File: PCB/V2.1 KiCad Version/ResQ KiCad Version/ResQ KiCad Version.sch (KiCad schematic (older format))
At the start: 7 parts, among them J1 Spare 1, J2 Spare 2, J3 OLED, J4 SD Card, J5 GPS, U1 WeMos_D1_mini

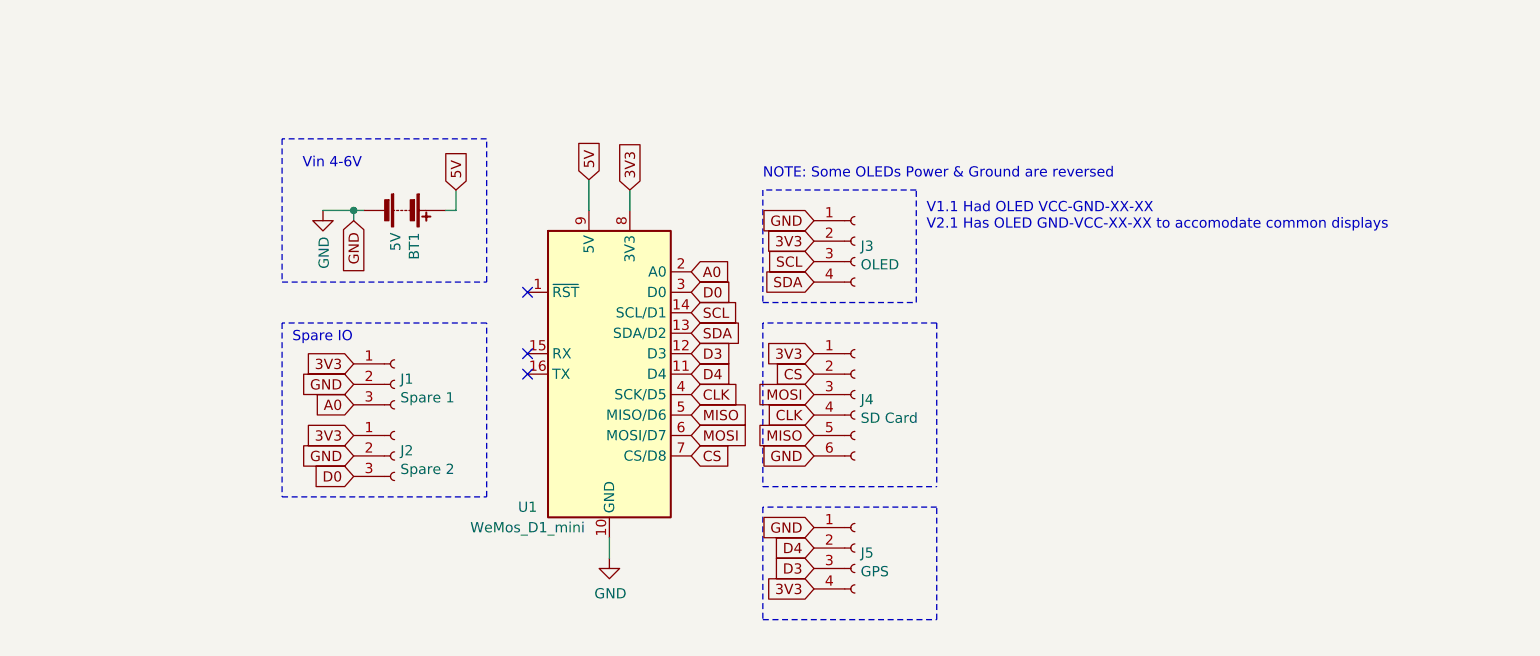
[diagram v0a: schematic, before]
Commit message: Purdier schematic
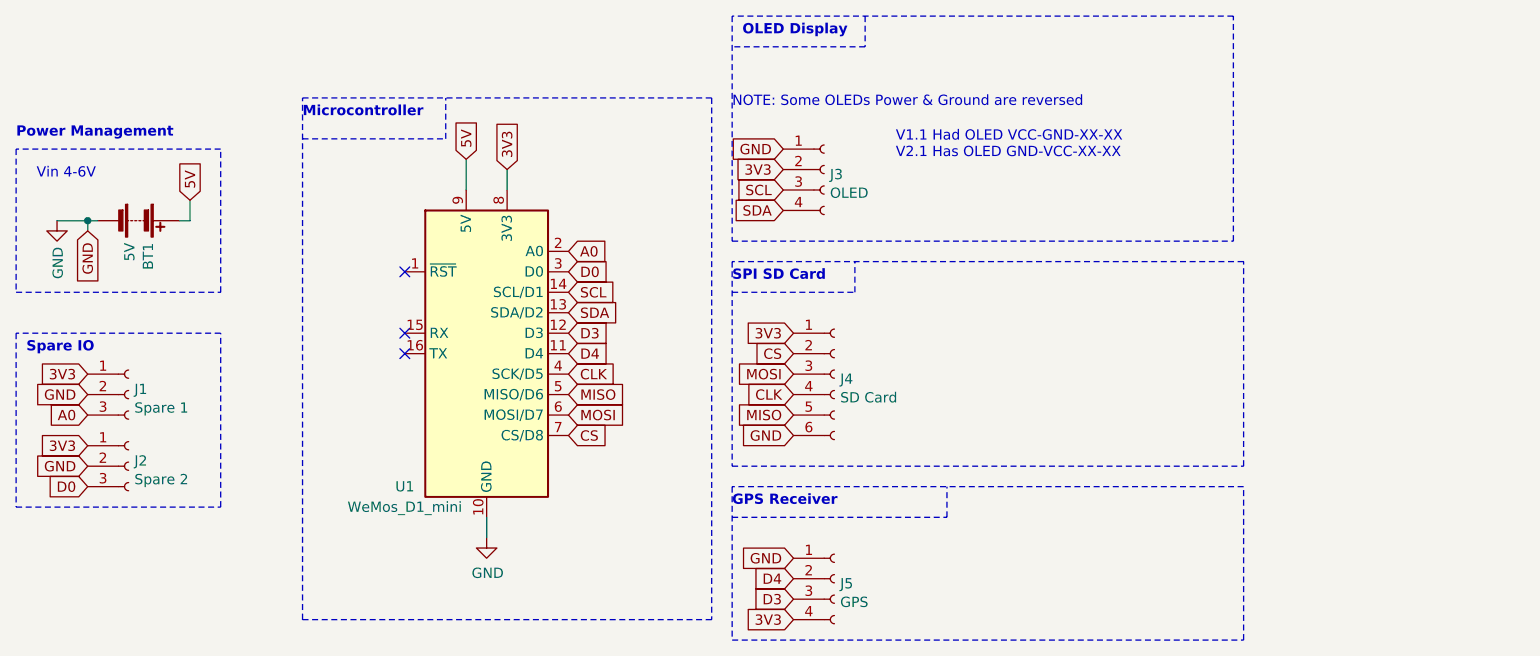
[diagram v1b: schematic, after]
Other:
- note added: "GPS Receiver"
- note added: "Microcontroller"
- note added: "OLED Display"
- note added: "Power Management"
- note added: "SPI SD Card"
- note added: "V1.1 Had OLED VCC-GND-XX-XX\nV2.1 Has OLED GND-VCC-XX-XX \n"
- note removed: "V1.1 Had OLED VCC-GND-XX-XX\nV2.1 Has OLED GND-VCC-XX-XX to accomodate common displays\n"
- moved on the sheet: BT1, J1, J2, J3, J4, J5, U1

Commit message: Purdy schematico
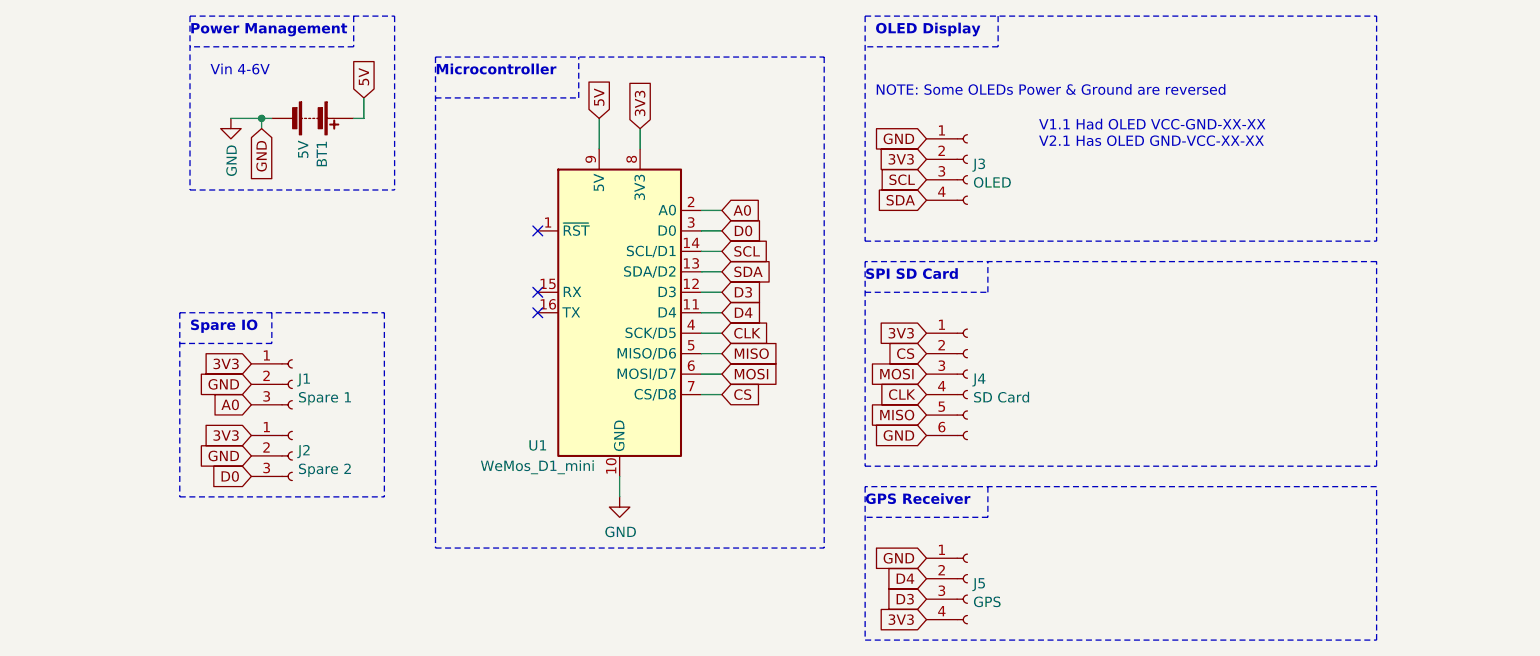
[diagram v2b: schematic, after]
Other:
- moved on the sheet: BT1, J1, J2, J3, J4, J5, U1
